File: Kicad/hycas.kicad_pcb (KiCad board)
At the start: 2 copper layers, 135.5 x 61.9 mm, 134 parts, among them J1 Conn_Coaxial, J2 S-Meter, J3 Vcc, J4 AGC Off, J5 Mute, J6 BFO, J7 Speaker, Q1 2N3904, Q10 2N3906, Q11 2N3904, Q12 2N3904, Q2 J310, Q3 2N3904, Q4 J310, Q5 2N3904, Q6 J310, Q7 2N3906, Q8 2N3906, Q9 2N3904, T1 16T 4T FB-43-2401, T2 T50-6, T3 T50-6, U1 LM324, U2 L7809, U3 TDA2003

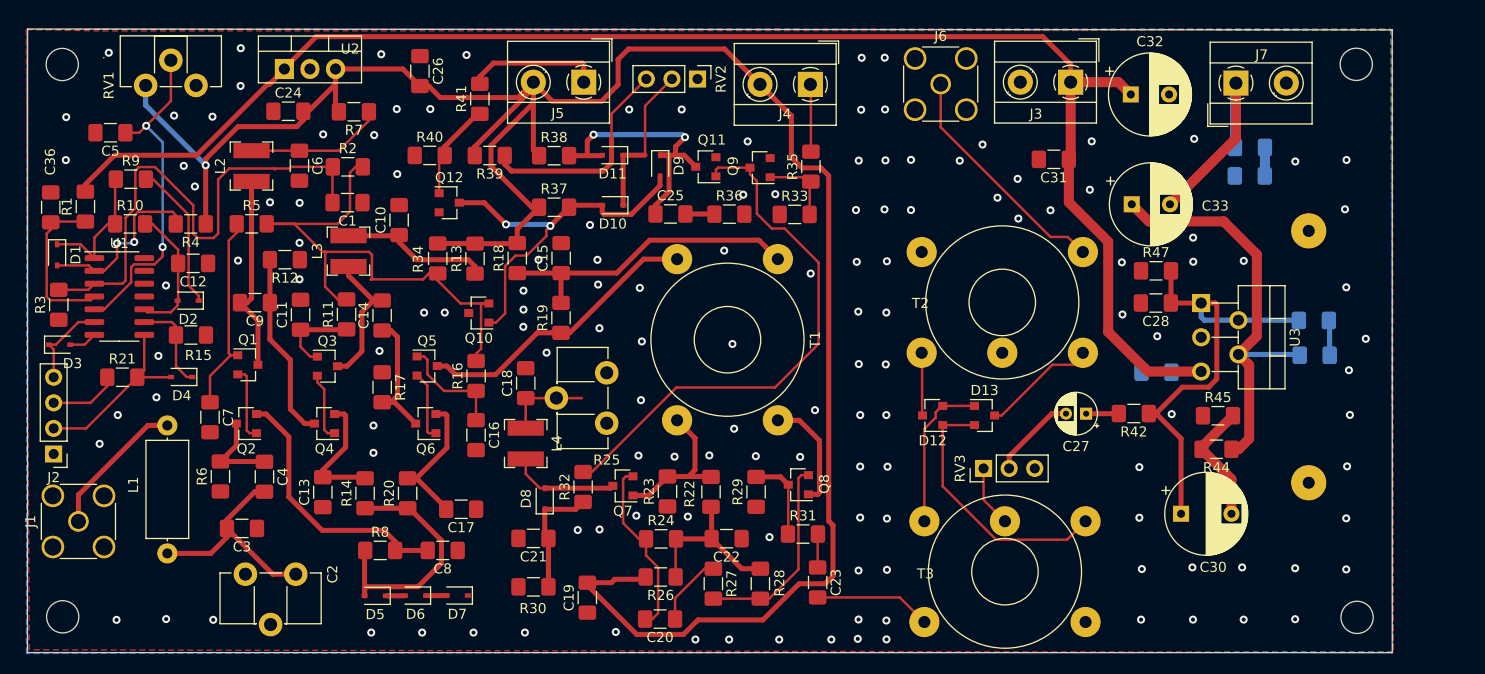
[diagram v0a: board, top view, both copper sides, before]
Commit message: Add files via upload
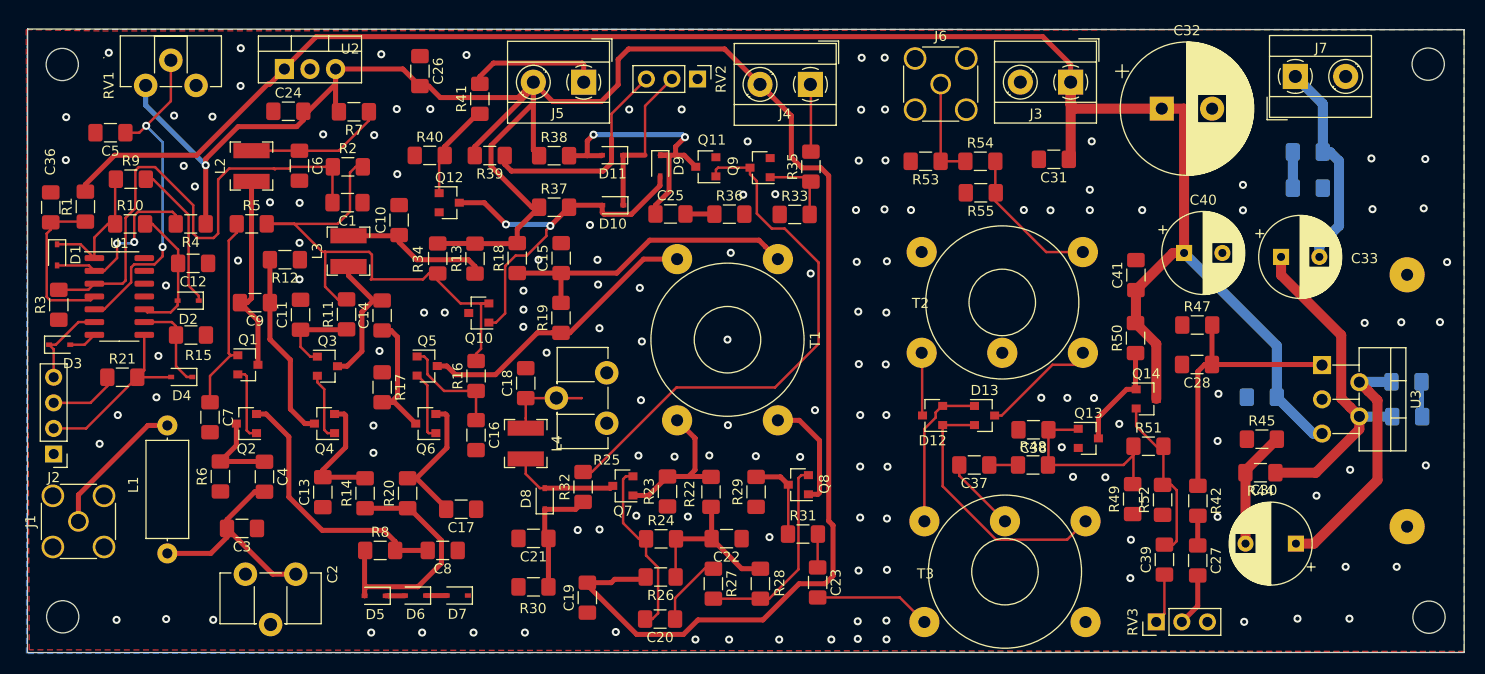
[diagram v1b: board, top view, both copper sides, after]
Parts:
- added C37: 1u, Capacitor_SMD:C_1206_3216Metric_Pad1.42x1.75mm_HandSolder, F.Cu at (135.8, 91.3)
- added C38: 100n, Capacitor_SMD:C_1206_3216Metric_Pad1.42x1.75mm_HandSolder, F.Cu at (141.7, 87.8)
- added C39: 1u, Capacitor_SMD:C_1206_3216Metric_Pad1.42x1.75mm_HandSolder, F.Cu at (154.7, 100.7)
- added C40: 470u, Capacitor_THT:CP_Radial_D8.0mm_P3.80mm, F.Cu at (156.6, 70.3)
- added C41: 100nf, Capacitor_SMD:C_1206_3216Metric_Pad1.42x1.75mm_HandSolder, F.Cu at (151.9, 72.5)
- added Q13: 2N3904_SOT23, Package_TO_SOT_SMD:SOT-23, F.Cu at (147.1, 88.7)
- added Q14: 2N3904_SOT23, Package_TO_SOT_SMD:SOT-23, F.Cu at (152.9, 84.8)
- added R48: 1k, Resistor_SMD:R_1206_3216Metric_Pad1.42x1.75mm_HandSolder, F.Cu at (141.6, 91.3)
- added R49: 1k, Resistor_SMD:R_1206_3216Metric_Pad1.42x1.75mm_HandSolder, F.Cu at (151.5, 94.7)
- added R50: 1k, Resistor_SMD:R_1206_3216Metric_Pad1.42x1.75mm_HandSolder, F.Cu at (151.8, 78.7)
- added R51: 5k, Resistor_SMD:R_1206_3216Metric_Pad1.42x1.75mm_HandSolder, F.Cu at (153.1, 89.5)
- added R52: 500, Resistor_SMD:R_1206_3216Metric_Pad1.42x1.75mm_HandSolder, F.Cu at (154.5, 94.8)
- added R53: 150, Resistor_SMD:R_1206_3216Metric_Pad1.42x1.75mm_HandSolder, F.Cu at (131.0, 61.2)
- added R54: 33, Resistor_SMD:R_1206_3216Metric_Pad1.42x1.75mm_HandSolder, F.Cu at (136.4, 61.2)
- added R55: 150, Resistor_SMD:R_1206_3216Metric_Pad1.42x1.75mm_HandSolder, F.Cu at (136.5, 64.3)
- C27: footprint Capacitor_THT:CP_Radial_D4.0mm_P2.00mm -> Capacitor_SMD:C_1206_3216Metric_Pad1.42x1.75mm_HandSolder
- C32: value 470u -> 2200u; footprint Capacitor_THT:CP_Radial_D8.0mm_P3.80mm -> Capacitor_THT:CP_Radial_D13.0mm_P5.00mm
- moved RV3 22.9 mm to (153.9, 106.9)
- moved C27 18.3 mm to (158.0, 100.8), turned to 270 degrees
- moved C33 15.7 mm to (166.3, 70.7)
- moved U3 13.5 mm to (170.3, 81.4)
- moved C30 11.8 mm to (167.7, 99.1), turned to 180 degrees
- moved R43 11.0 mm to (178.7, 83.1)
- moved C29 11.0 mm to (178.8, 86.5)
- moved R42 10.7 mm to (158.0, 94.9), turned to 270 degrees
- moved C35 10.7 mm to (164.4, 84.6)
- moved   10.7 mm to (178.8, 97.5)
- moved   10.7 mm to (178.8, 72.5)
- moved C28 7.35 mm to (157.9, 81.4)
- moved   7.14 mm to (181.0, 106.4)
- moved   7.14 mm to (180.9, 51.5)
- moved R47 6.76 mm to (157.9, 77.4)
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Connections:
- C30 pad 1: Net-(C28-Pad1) -> Net-(C30-Pad1)
- Q7 pad 1: Vin2 -> Net-(Q7-Pad1)
- R43 pad 1: Net-(C28-Pad1) -> Net-(C30-Pad1)
- RV3 pad 1: Net-(RV3-Pad1) -> Net-(C39-Pad1)
- T2 pad 1: Net-(J6-Pad1) -> Net-(R54-Pad2)
- T3 pad 4: Net-(RV3-Pad1) -> Net-(C37-Pad2)
- U3 pad 2: Net-(C28-Pad1) -> Net-(C30-Pad1)
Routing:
- net V12v: track 154.3 -> 185.4 mm
- net Net-(C30-Pad1): track 0.00 -> 24.4 mm
- net Net-(C38-Pad1): track 0.00 -> 20.1 mm
- net Net-(C28-Pad1): track 45.6 -> 27.9 mm
- net Net-(C39-Pad2): track 0.00 -> 17.2 mm
- net Net-(R54-Pad2): track 0.00 -> 14.7 mm
- net Net-(J6-Pad1): track 23.5 -> 10.1 mm
- net Net-(Q13-Pad3): track 0.00 -> 10.6 mm
- net Net-(C29-Pad2): track 42.3 -> 33.7 mm
- net Net-(C37-Pad2): track 0.00 -> 7.47 mm
- net Net-(RV3-Pad1): track 6.12 -> 0.00 mm
- net Net-(C39-Pad1): track 0.00 -> 5.03 mm
- net Net-(C27-Pad2): track 8.60 -> 5.27 mm
- net Net-(C37-Pad1): track 0.00 -> 2.86 mm
- net Net-(C34-Pad1): track 2.83 -> 3.58 mm
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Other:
- board size 135.5 x 61.9 mm -> 142.6 x 61.9 mm

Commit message: updated version
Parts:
- R9: value 22k -> 4.7k
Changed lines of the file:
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@@
       (effects (font (size 1 1) (thickness 0.15)))
     )
-    (fp_text value 22k (at 0 1.82) (layer F.Fab)
+    (fp_text value 4.7k (at 0 1.82) (layer F.Fab)
       (effects (font (size 1 1) (thickness 0.15)))
     )
@@
   (segment (start 169.53906 99.14128) (end 175.837481 92.842859) (width 1) (layer F.Cu) (net 81))
   (segment (start 167.73906 99.14128) (end 169.53906 99.14128) (width 1) (layer F.Cu) (net 81))
-  (segment (start 151.59322 89.45372) (end 151.61354 89.47404) (width 0.25) (layer F.Cu) (net 83))
   (segment (start 137.90582 64.27724) (end 137.94646 64.31788) (width 0.25) (layer F.Cu) (net 82))
   (segment (start 137.90582 61.19114) (end 137.90582 64.27724) (width 0.25) (layer F.Cu) (net 82))
@@
   (segment (start 137.94646 65.19288) (end 142.9541 70.20052) (width 0.25) (layer F.Cu) (net 82))
   (segment (start 137.94646 64.31788) (end 137.94646 65.19288) (width 0.25) (layer F.Cu) (net 82))
+  (segment (start 151.59322 89.45372) (end 151.61354 89.47404) (width 0.25) (layer F.Cu) (net 83))
   (segment (start 143.17632 91.29014) (end 143.13314 91.33332) (width 0.25) (layer F.Cu) (net 83))
   (segment (start 143.17632 87.84082) (end 143.17632 91.29014) (width 0.25) (layer F.Cu) (net 83))
